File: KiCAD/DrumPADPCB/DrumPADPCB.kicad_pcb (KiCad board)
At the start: 2 copper layers, 24 parts, among them J1 Conn_01x02_Pin, J3 Conn_01x04_Pin, U1 LM321, U2 LM321

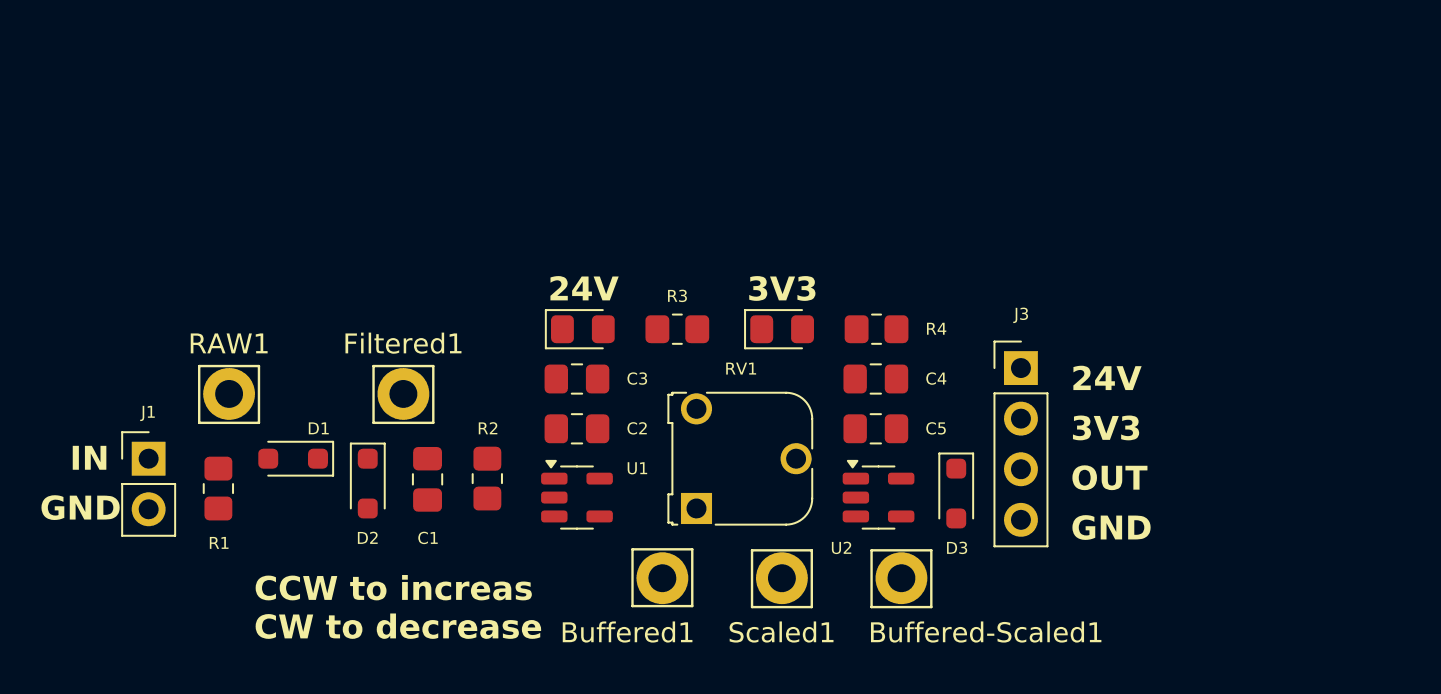
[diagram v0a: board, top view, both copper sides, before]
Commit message: PCB V1.0 release ready to order
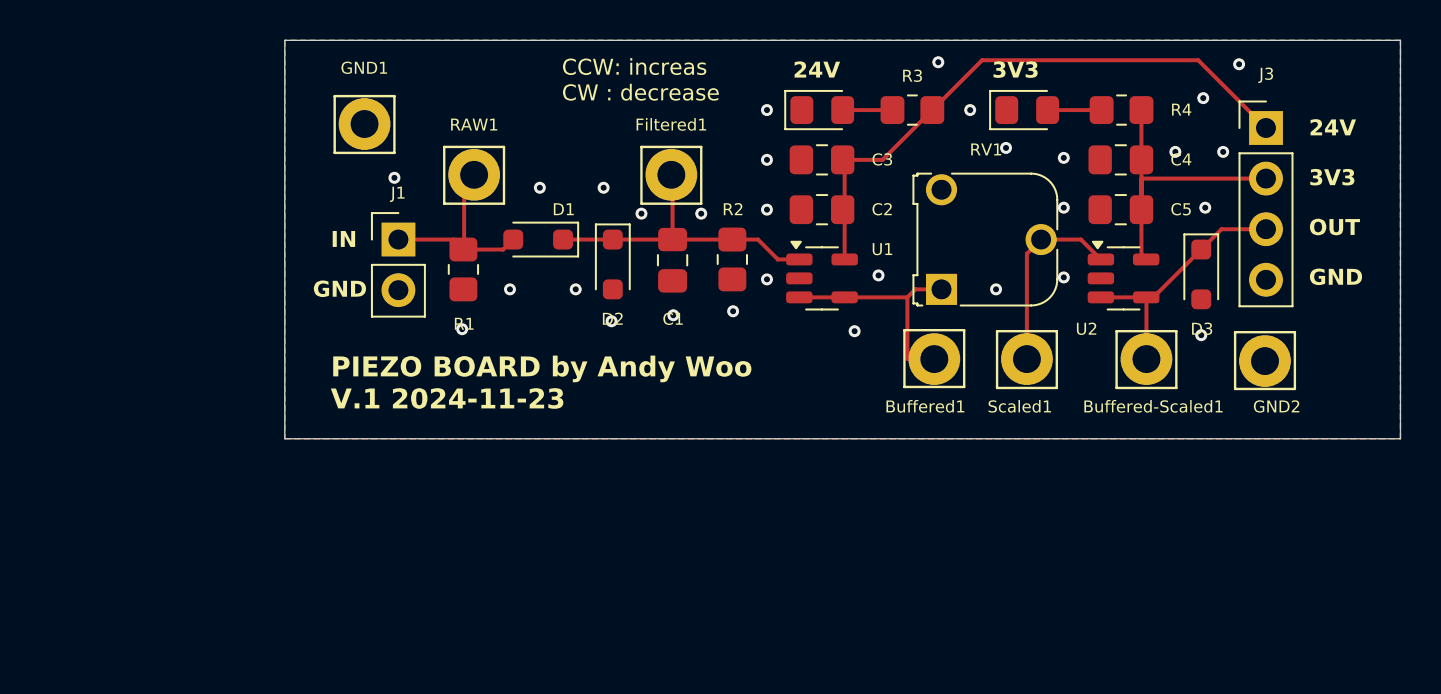
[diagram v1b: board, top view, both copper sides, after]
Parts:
- added GND1: TestPoint, Connector_Pin:Pin_D1.4mm_L8.5mm_W2.8mm_FlatFork, F.Cu at (84.3, 58.2)
- added GND2: TestPoint, Connector_Pin:Pin_D1.4mm_L8.5mm_W2.8mm_FlatFork, F.Cu at (129.5, 70.1)
- moved Buffered1 17.5 mm to (112.9, 70.0)
- moved Filtered1 17.4 mm to (99.7, 60.8)
- moved J3 17.2 mm to (129.6, 58.4)
- moved J1 16.7 mm to (86.0, 64.0)
- moved U2 16.5 mm to (122.4, 66.0)
- moved Buffered-Scaled1 16.5 mm to (123.5, 70.0)
- moved C1 16.5 mm to (99.8, 65.0)
- moved C2 16.5 mm to (107.3, 62.5)
- moved C3 16.5 mm to (107.3, 60.0)
- moved C4 16.5 mm to (122.3, 60.0)
- moved C5 16.5 mm to (122.3, 62.5)
- moved D1 16.5 mm to (93.0, 64.0)
- moved D2 16.5 mm to (96.8, 65.2)
- moved D3 16.5 mm to (126.3, 65.8)
- moved D5 16.5 mm to (117.6, 57.5)
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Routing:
- net 24V: track 0.00 -> 29.3 mm
- net Net-(D1-K): track 0.00 -> 16.2 mm
- net 3V3: track 0.00 -> 15.4 mm
- net /Piezo Processing Board/Sig_Out: track 0.00 -> 12.8 mm
- net Net-(U1--): track 0.00 -> 10.4 mm
- net Net-(D1-A): track 0.00 -> 10.4 mm
- net Net-(U2-+): track 0.00 -> 9.71 mm
- net Net-(D5-A): track 0.00 -> 2.72 mm
- net Net-(D4-A): track 0.00 -> 2.50 mm
- net GND: vias 0 -> 30
- added copper zone on B.Cu, net GND
- added copper zone on F.Cu, net GND
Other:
- board outline added: 56 x 20 mm
- board text added: "CCW: increas CW : decrease"
- board text added: "PIEZO BOARD by Andy Woo V.1 2024-11-23"
- board text removed: "CCW to increas CW to decrease"
